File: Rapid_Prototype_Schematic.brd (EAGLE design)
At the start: 142 x 95 mm, 177 parts, among them IC2 SI4459ADY-T1-GE3, IC8 SI4485DY-T1-GE3, J1 XT60-M, J10 XT60-M, J2 XT60-M, J3 Vertical Qwiic Connector, J4 UJ2-MIBH-2-SMT-TR-67, J5 XT60-M, J6 XT60-M, J7 XT60-M, J8 XT60-M, J9 XT60-M, Q1 LTV-8141S, Q10 SI4435DDY, Q11 DMN65D8LFB-7, Q12 SI4435DDY, Q13 DMN65D8LFB-7, Q14 SI4435DDY, Q15 DMN65D8LFB-7, Q16 2N7002PW, Q2 2N7002PW, Q3 DMN65D8LFB-7, Q4 SI4435DDY, Q5 DMN65D8LFB-7, Q6 SI4435DDY, Q7 DMN65D8LFB-7, Q8 SI4435DDY, Q9 DMN65D8LFB-7, U1 LM35DM, U2 LM2904ITPX/NOPB, U3 LM2904ITPX/NOPB, U4 LM2904ITPX/NOPB, U5 LM2904ITPX/NOPB, U6 LM2904ITPX/NOPB, U7 TLV1117LV33DCYR, U8 LT1374IS8-5PBF

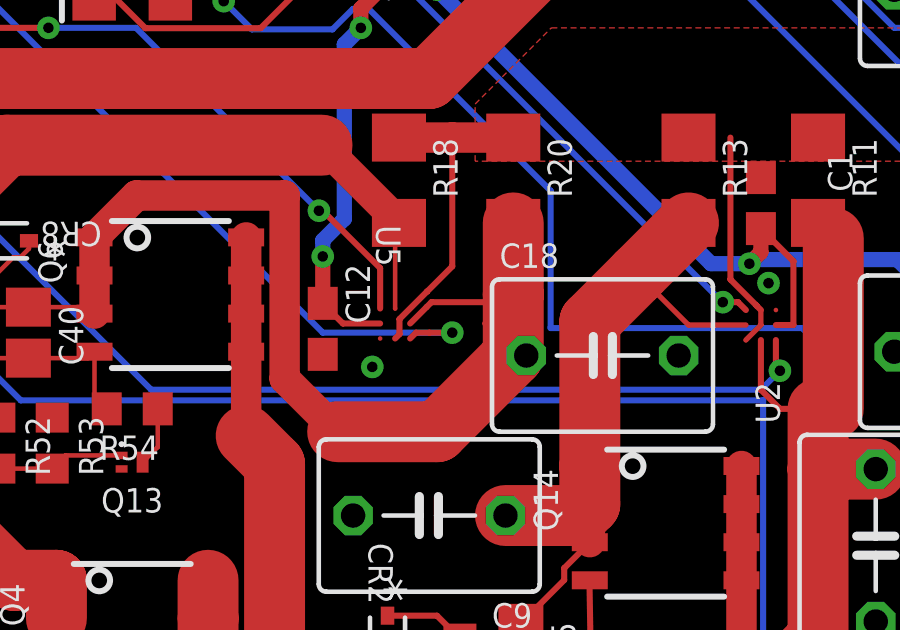
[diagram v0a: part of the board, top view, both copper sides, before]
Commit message: Update Rapid_Prototype_Schematic.brd
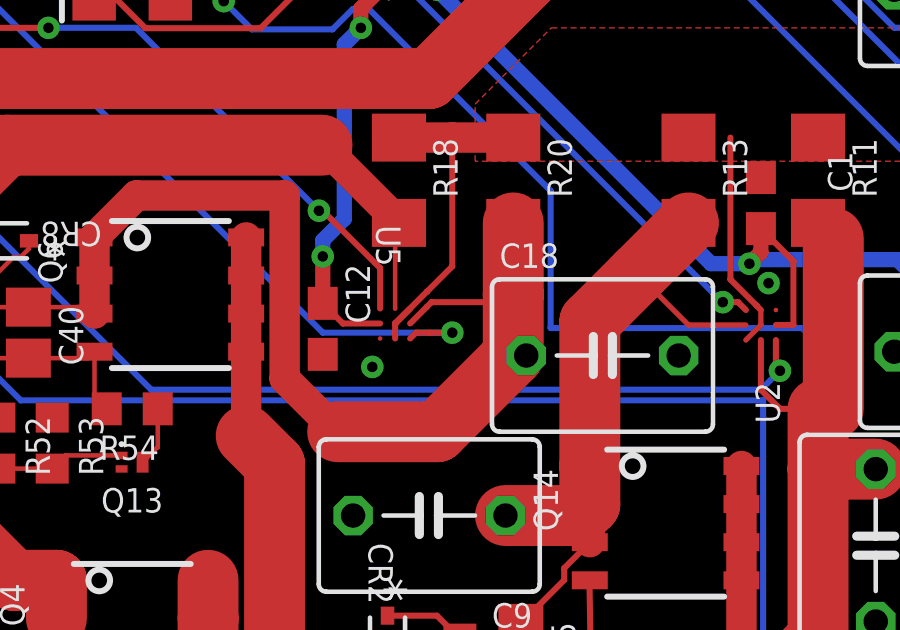
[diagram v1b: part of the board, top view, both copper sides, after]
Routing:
- net ESC_PF_POWER: track 42.4 -> 41.4 mm
- net ESC_POWER: track 33.8 -> 34.6 mm
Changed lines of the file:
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@@
 <vertex x="66.04" y="77.47"/>
 </polygon>
-<wire x1="60.9774" y1="67.259203125" x2="60.833" y2="67.114803125" width="0.2032" layer="1"/>
-<wire x1="60.9774" y1="67.76210625" x2="60.9774" y2="67.259203125" width="0.2032" layer="1"/>
 <wire x1="62.738" y1="69.519803125" x2="61.899796875" y2="68.6816" width="0.2032" layer="1"/>
 <wire x1="61.899796875" y1="68.6816" x2="61.89689375" y2="68.6816" width="0.2032" layer="1"/>
-<wire x1="61.89689375" y1="68.6816" x2="60.9774" y2="67.76210625" width="0.2032" layer="1"/>
-<wire x1="60.833" y1="67.114803125" x2="61.333" y2="68.114803125" width="0" layer="19" extent="1-1"/>
+<wire x1="61.89689375" y1="68.6816" x2="60.833" y2="67.61770625" width="0.2032" layer="1"/>
+<wire x1="60.833" y1="67.61770625" x2="60.833" y2="67.114803125" width="0.2032" layer="1"/>
+<wire x1="61.333" y1="68.114803125" x2="60.835903125" y2="67.61770625" width="0.2032" layer="1"/>
+<wire x1="60.835903125" y1="67.61770625" x2="60.833" y2="67.61770625" width="0.2032" layer="1"/>
 </signal>
 <signal name="N$1">
@@
 <wire x1="64.77" y1="68.58" x2="64.77" y2="70.968" width="2.032" layer="1"/>
 <wire x1="64.77" y1="68.58" x2="64.516" y2="68.326" width="0.1524" layer="1"/>
-<wire x1="64.516" y1="68.326" x2="63.804803125" y2="67.614803125" width="0.1524" layer="1"/>
 <wire x1="64.77" y1="66.548" x2="65.2043375" y2="66.548" width="1.016" layer="1"/>
 <wire x1="64.77" y1="66.548" x2="62.23" y2="64.008" width="2.032" layer="1"/>

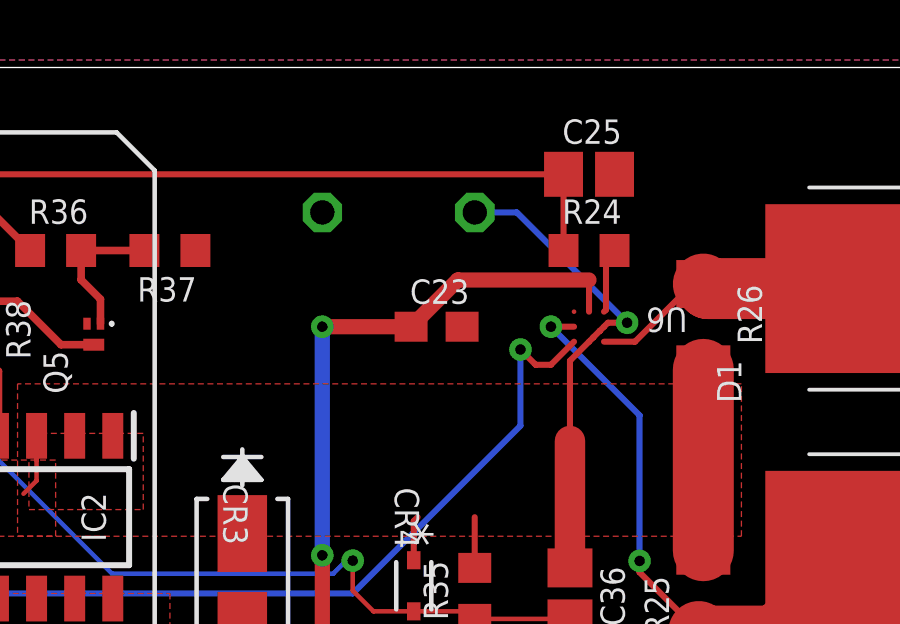
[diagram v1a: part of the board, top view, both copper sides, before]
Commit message: Update Rapid_Prototype_Schematic.brd
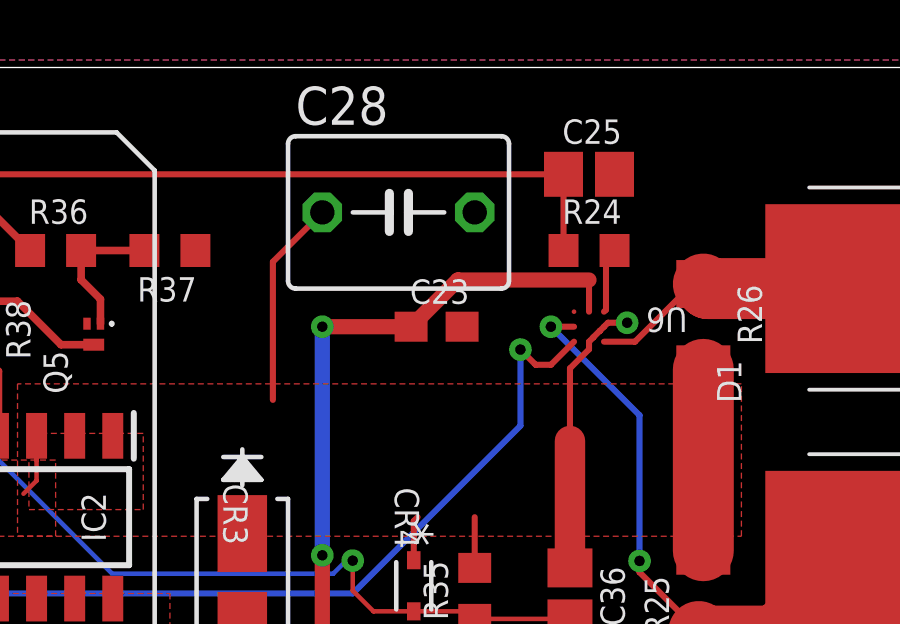
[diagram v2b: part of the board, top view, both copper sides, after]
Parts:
- flipped C28 to the top
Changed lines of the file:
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@@
 <attribute name="VALUE" x="83.185" y="80.899" size="1.27" layer="27" ratio="10" rot="R180"/>
 </element>
-<element name="C28" library="adafruit" library_urn="urn:adsk.eagle:library:420" package="C050-050X075" package3d_urn="urn:adsk.eagle:package:6240360/1" value="220µF" x="99.06" y="90.17" smashed="yes" rot="MR0">
-<attribute name="NAME" x="102.489" y="93.091" size="1.27" layer="26" ratio="10" rot="MR0"/>
-<attribute name="VALUE" x="102.235" y="88.011" size="1.27" layer="28" ratio="10" rot="MR0"/>
+<element name="C28" library="adafruit" library_urn="urn:adsk.eagle:library:420" package="C050-050X075" package3d_urn="urn:adsk.eagle:package:6240360/1" value="220µF" x="99.06" y="90.17" smashed="yes">
+<attribute name="NAME" x="95.631" y="93.091" size="1.27" layer="25" ratio="10"/>
+<attribute name="VALUE" x="95.885" y="88.011" size="1.27" layer="27" ratio="10"/>
 </element>
 <element name="C29" library="adafruit" library_urn="urn:adsk.eagle:library:420" package="C1206" package3d_urn="urn:adsk.eagle:package:6240335/1" value="22uF" x="34.417" y="17.78" smashed="yes" rot="R90">
@@
 <wire x1="82.484" y1="89.789" x2="82.484" y2="86.03315" width="0.2032" layer="1"/>
 <wire x1="104.775" y1="82.55" x2="104.775" y2="78.32" width="1.016" layer="1"/>
-<wire x1="105.41" y1="85.86" x2="104.775" y2="85.225" width="0.2032" layer="1"/>
-<wire x1="104.775" y1="85.225" x2="104.775" y2="82.55" width="0.2032" layer="1"/>
+<wire x1="105.41" y1="85.86" x2="105.41" y2="85.606" width="0.2032" layer="1"/>
+<wire x1="105.41" y1="85.606" x2="104.775" y2="84.971" width="0.2032" layer="1"/>
+<wire x1="104.775" y1="84.971" x2="104.775" y2="82.55" width="0.2032" layer="1"/>
 <wire x1="105.91" y1="86.36" x2="105.7656" y2="86.2156" width="0.2032" layer="1"/>
 <wire x1="105.7656" y1="86.2156" x2="105.7627" y2="86.2156" width="0.2032" layer="1"/>
@@
 <wire x1="106.0422" y1="86.4922" x2="106.68" y2="86.4922" width="0.2032" layer="1"/>
 <via x="106.68" y="86.4922" extent="1-16" drill="0.35"/>
-<wire x1="106.68" y1="86.4922" x2="103.0022" y2="90.17" width="0.2032" layer="16"/>
-<wire x1="103.0022" y1="90.17" x2="101.6" y2="90.17" width="0.2032" layer="16"/>
 <wire x1="86.55896875" y1="80.7911" x2="86.995" y2="81.22713125" width="0.1524" layer="1"/>
 <wire x1="86.995" y1="81.22713125" x2="86.995" y2="82.722" width="0.1524" layer="1"/>
@@
 <vertex x="87.63" y="79.375"/>
 </polygon>
+<wire x1="96.52" y1="90.17" x2="94.8718" y2="88.5218" width="0.2032" layer="1"/>
+<wire x1="94.8718" y1="88.5218" x2="94.8718" y2="83.919359375" width="0.2032" layer="1"/>
 </signal>
 <signal name="N$3">
